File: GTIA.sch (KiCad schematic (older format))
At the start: 72 parts, among them J2 Video, Q1 2N3904, Q2 2N3904, Q3 2N3904, Q6 2N3904, U17 GTIA, U18 74LS08, U20 4050, U21 74LS74, Y2 4,43 MHz

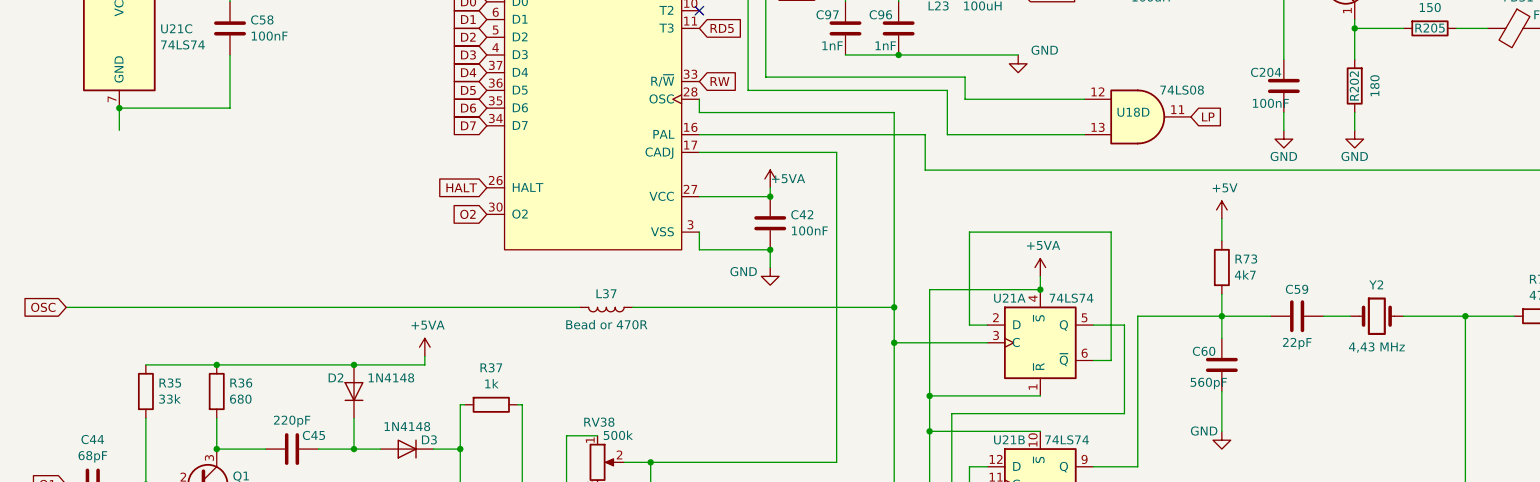
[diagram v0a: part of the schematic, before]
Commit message: Patching
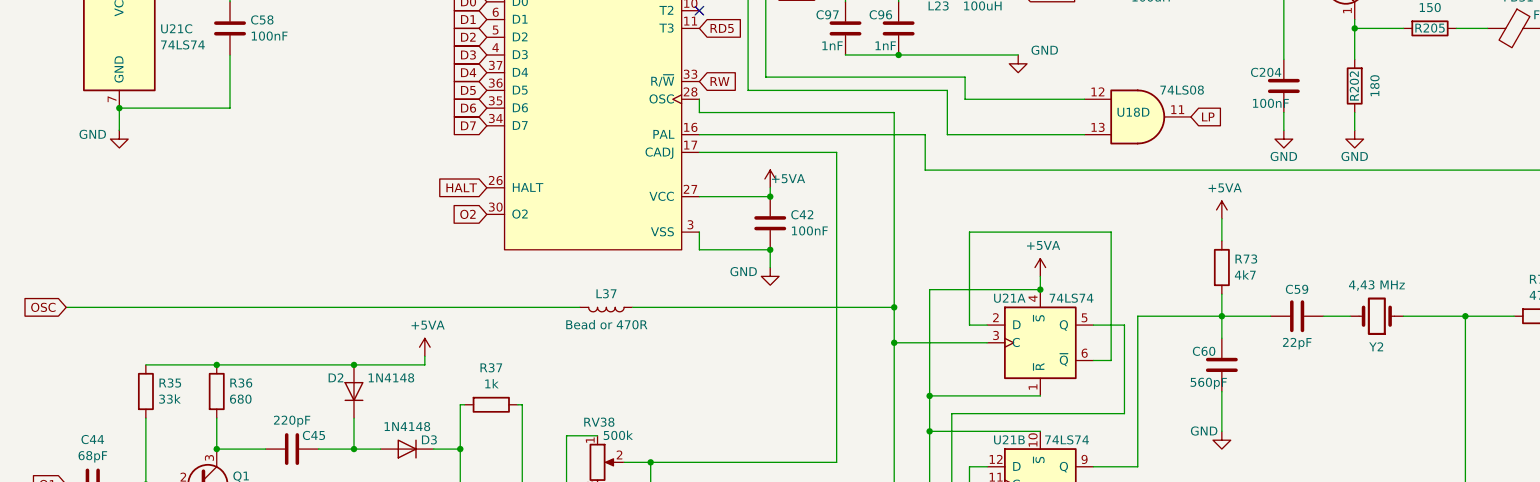
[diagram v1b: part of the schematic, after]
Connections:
- net +5V: no longer R73.1
- net +5VA: now also R73.1
- net GND: now also C58.2, U21.7 (GND)
- net at C59.2: now also Y2.2; no longer Y2.1
- net at C111.1, L8.1, R71.2: now also Y2.1; no longer Y2.2
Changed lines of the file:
@@
 F 3 "~" H 8150 5250 50  0001 C CNN
 	1    8150 5250
-	1    0    0    -1
+	-1   0    0    1
 $EndComp
 $Comp
@@
 $EndComp
 $Comp
-L power:+5V #PWR0166
-U 1 1 602CB043
-P 7275 4700
-F 0 "#PWR0166" H 7275 4550 50  0001 C CNN
-F 1 "+5V" H 7290 4873 50  0000 C CNN
-F 2 "" H 7275 4700 50  0001 C CNN
-F 3 "" H 7275 4700 50  0001 C CNN
-	1    7275 4700
-	1    0    0    -1
-$EndComp
-$Comp
 L Device:C C204
 U 1 1 60308154
@@
 Wire Wire Line
 	3325 6225 3325 6250
+$Comp
+L power:GND #PWR0249
+U 1 1 6034B9B1
+P 1050 4200
+F 0 "#PWR0249" H 1050 3950 50  0001 C CNN
+F 1 "GND" H 900 4175 50  0000 C CNN
+F 2 "" H 1050 4200 50  0001 C CNN
+F 3 "" H 1050 4200 50  0001 C CNN
+	1    1050 4200
+	1    0    0    -1
+$EndComp
+$Comp
+L power:+5VA #PWR0166
+U 1 1 6035DAC7
+P 7275 4700
+F 0 "#PWR0166" H 7275 4550 50  0001 C CNN
+F 1 "+5VA" H 7290 4873 50  0000 C CNN
+F 2 "" H 7275 4700 50  0001 C CNN
+F 3 "" H 7275 4700 50  0001 C CNN
+	1    7275 4700
+	1    0    0    -1
+$EndComp
 $EndSCHEMATC
